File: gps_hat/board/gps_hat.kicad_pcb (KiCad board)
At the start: 2 copper layers, 12 parts, among them IC1 MTK3339, J1 Conn_02x10_Odd_Even, J2 U.FL-R-SMT(10)

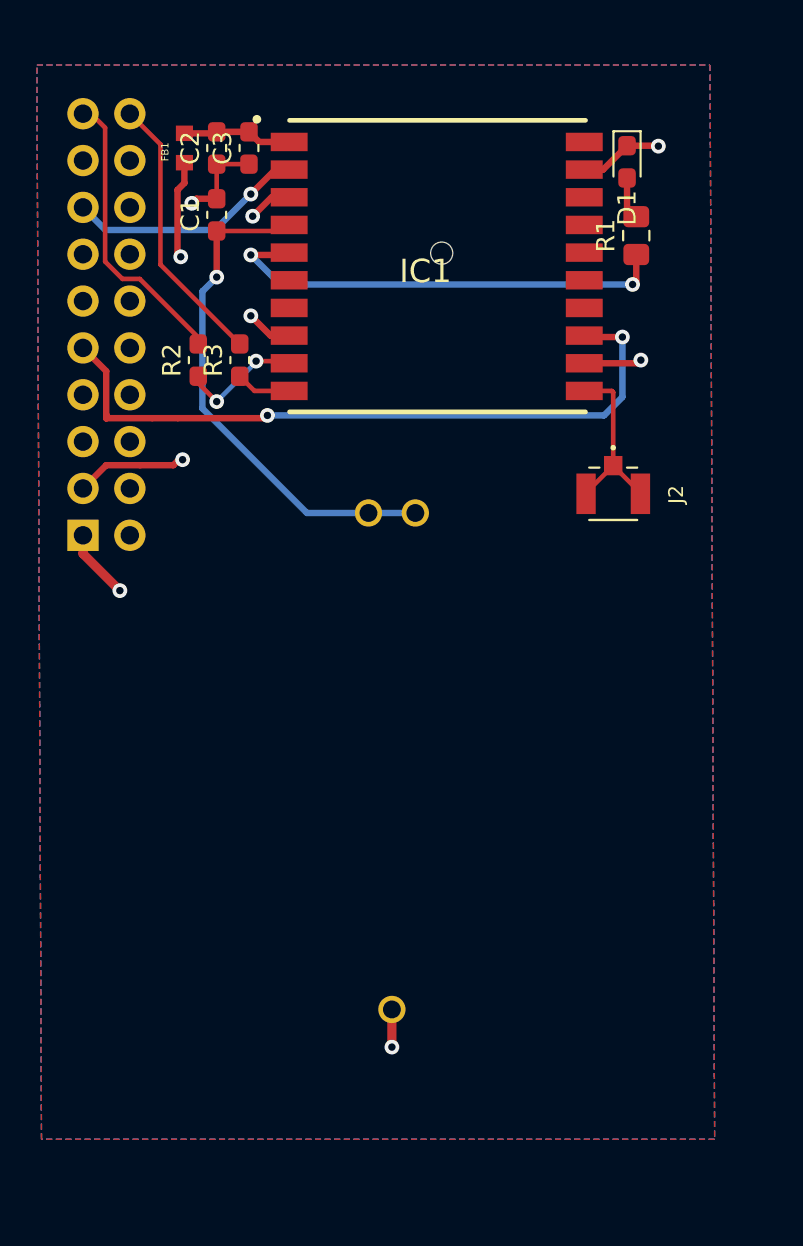
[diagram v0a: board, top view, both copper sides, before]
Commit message: Last Revision
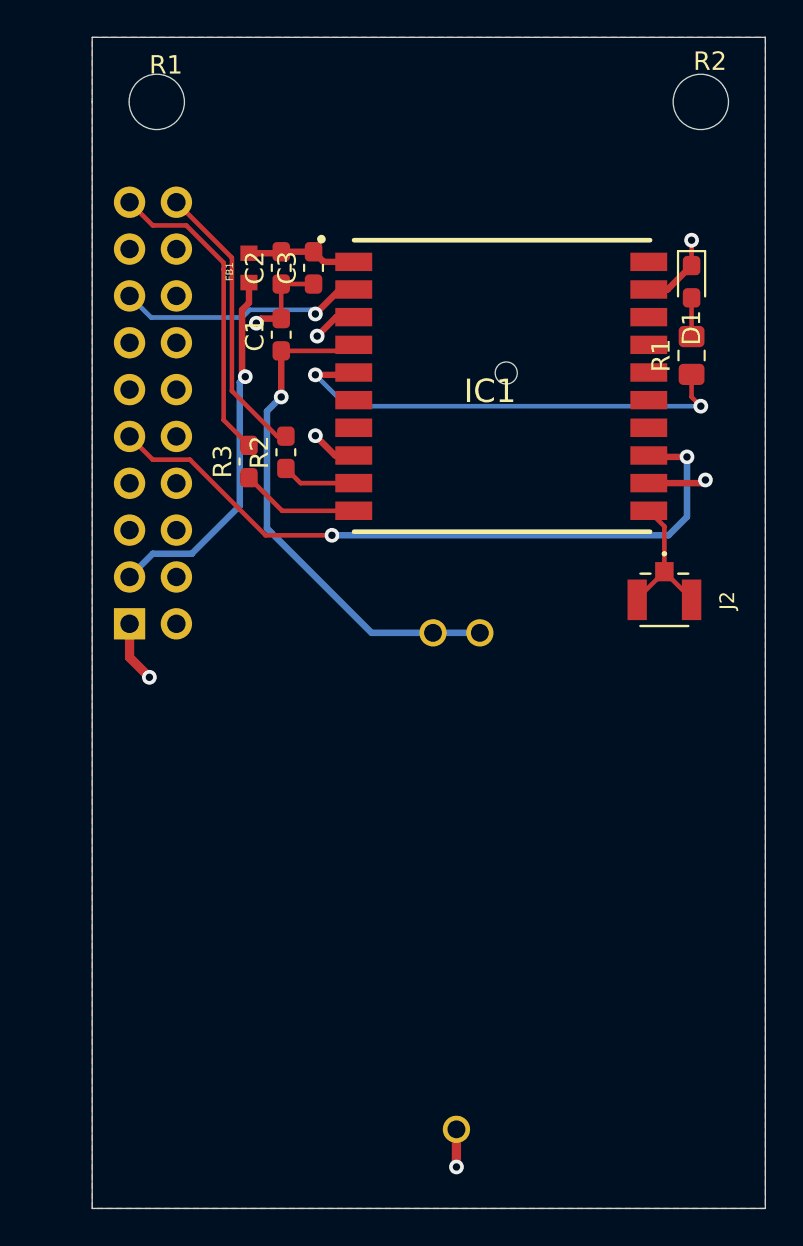
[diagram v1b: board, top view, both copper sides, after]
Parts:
- added R1: MountingHole, MountingHole:MountingHole_3mm, F.Cu at (133.0, 60.0)
- added R2: MountingHole, MountingHole:MountingHole_3mm, F.Cu at (162.5, 60.0)
- moved BT1 7.38 mm to (149.2, 102.2)
- moved C1 7.38 mm to (139.8, 72.6)
- moved C2 7.38 mm to (139.8, 69.0)
- moved C3 7.38 mm to (141.5, 69.0)
- moved D1 7.38 mm to (162.0, 69.8)
- moved FB1 7.38 mm to (138.0, 69.0)
- moved IC1 7.38 mm to (159.8, 67.5)
- moved R1 7.16 mm to (162.0, 73.8)
- moved R2 6.90 mm to (140.0, 79.0)
- moved J2 6.38 mm to (160.5, 87.0)
- moved R3 5.52 mm to (138.0, 79.5)
- moved J1 5.42 mm to (131.5, 88.3)
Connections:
- J1 pad 19: /RX -> /TX
- J1 pad 20: /TX -> /RX
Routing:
- net +3V3: track 11.4 -> 20.0 mm, vias 2 -> 1
- net Net-(IC1-Pad10): track 3.47 -> 6.89 mm
- net Net-(IC1-Pad9): track 6.71 -> 4.01 mm, vias 2 -> 0
- net /TX: track 15.0 -> 16.9 mm
- net Net-(IC1-Pad11): track 9.85 -> 7.92 mm
- net GND: track 23.6 -> 22.8 mm
- net Net-(IC1-Pad5): track 25.2 -> 25.8 mm
- removed copper zone on B.Cu, net +3V3
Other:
- board outline added: 36.5 x 63.5 mm
